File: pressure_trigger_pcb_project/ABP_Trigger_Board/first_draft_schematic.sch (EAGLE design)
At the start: 28 parts, among them U1 OPA4340UA

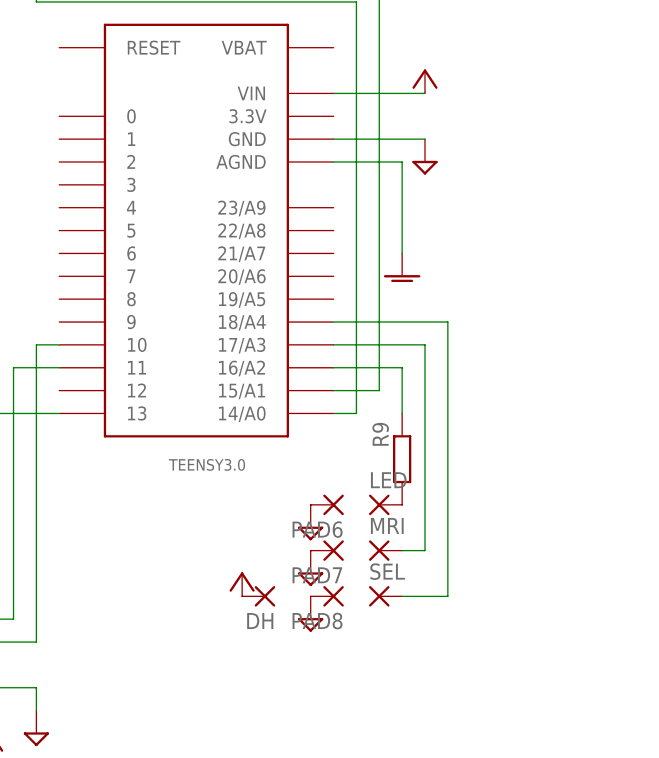
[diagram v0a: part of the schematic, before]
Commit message: schematic before package switch
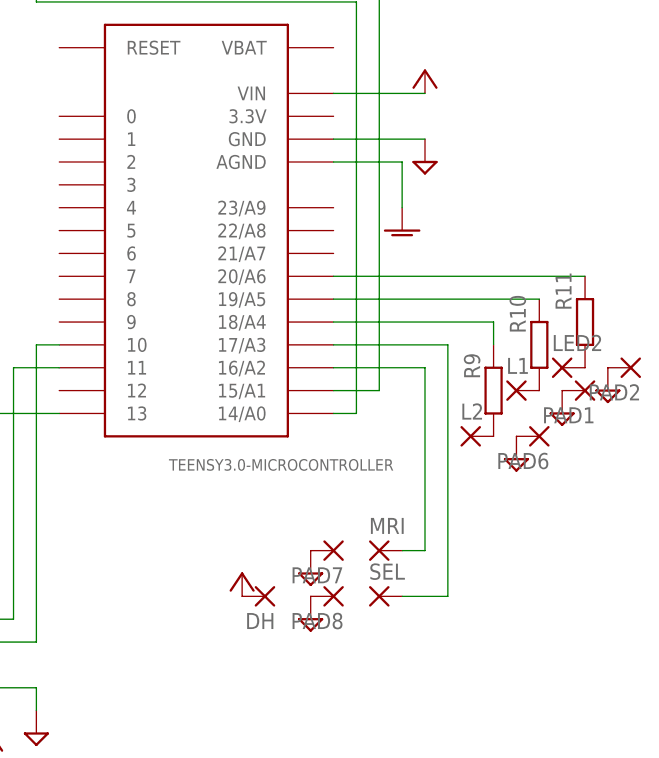
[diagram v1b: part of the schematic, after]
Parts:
- removed LED: WIREPAD1,6/0,9, wirepad:WIREPAD1,6/0,9
- added L1, L2, LED2, PAD1, PAD2: WIREPAD1,6/0,9, wirepad:WIREPAD1,6/0,9
- added R10, R11: 681, resistor:R-EU_R0805
- renumbered TEENSY3.0 to TEENSY3.0-MICROCONTROLLER
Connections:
- new net N$18: L1.P, R10.1
- new net N$21: R10.2, TEENSY3.0-MICROCONTROLLER.19/A5
- new net N$22: LED2.P, R11.1
- new net N$23: R11.2, TEENSY3.0-MICROCONTROLLER.20/A6
- net GND: now also PAD1.P, PAD2.P
- net N$11: now also L2.P; no longer LED.P
- net N$14: now also TEENSY3.0-MICROCONTROLLER.18/A4; no longer TEENSY3.0-MICROCONTROLLER.16/A2
- net N$15: now also TEENSY3.0-MICROCONTROLLER.16/A2; no longer TEENSY3.0-MICROCONTROLLER.17/A3
- net N$16: now also TEENSY3.0-MICROCONTROLLER.17/A3; no longer TEENSY3.0-MICROCONTROLLER.18/A4
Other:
- moved on the sheet: PAD6, R9
